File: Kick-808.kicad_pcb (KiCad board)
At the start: 2 copper layers, 19.3 x 106.5 mm, 70 parts, among them J3 Conn_02x05_Odd_Even, Q1 BC847, Q2 BC847, Q3 BC857, Q4 BC847, Q5 BC847, Q6 BC847, Q7 BC847, SW1 SW_Push_LED, U1 TL072, U2 TL072

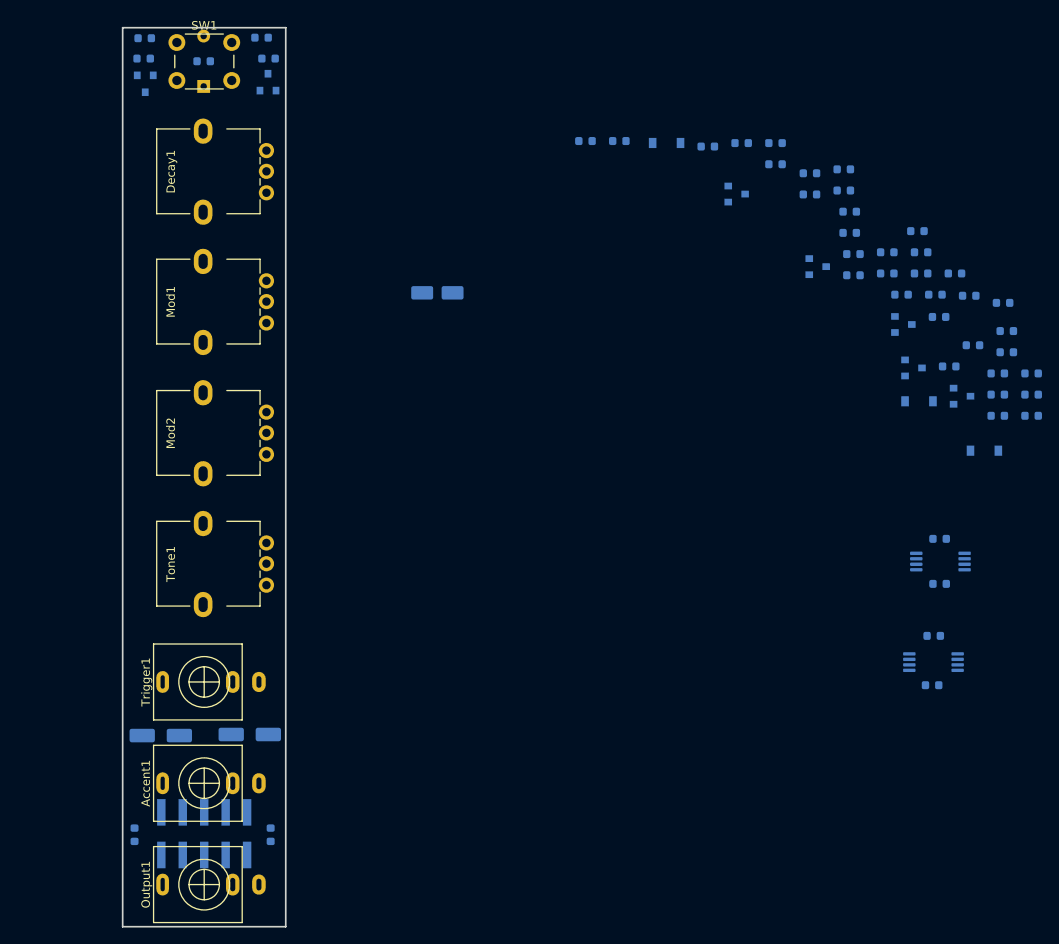
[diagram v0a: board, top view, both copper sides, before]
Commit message: Outline placement.
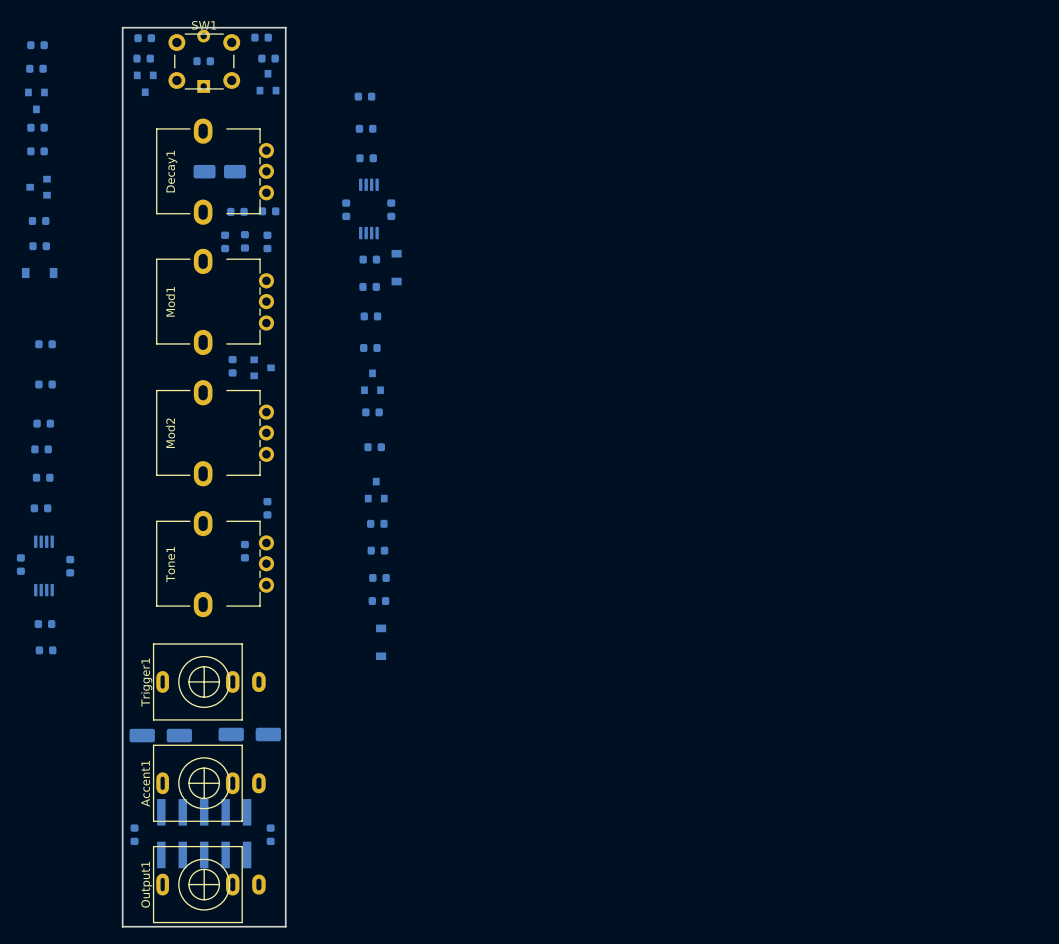
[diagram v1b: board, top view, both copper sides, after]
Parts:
- moved R15 119.8 mm to (107.4, 71.2), turned to 180 degrees
- moved R30 118.4 mm to (108.1, 119.0)
- moved R4 117.6 mm to (107.7, 98.3), turned to 180 degrees
- moved R11 116.5 mm to (107.7, 105.3)
- moved D2 113.9 mm to (107.5, 77.4)
- moved C2 111.0 mm to (107.3, 63.0), turned to 180 degrees
- moved R3 110.7 mm to (108.0, 95.2), turned to 180 degrees
- moved C14 108.9 mm to (105.3, 112.0), turned to 270 degrees
- moved R12 108.2 mm to (107.3, 60.2)
- moved U1 106.0 mm to (108.0, 112.1), turned to 270 degrees
- moved C11 105.5 mm to (108.3, 122.1), turned to 180 degrees
- moved C8 104.5 mm to (107.5, 74.2), turned to 180 degrees
- moved Q4 103.7 mm to (107.4, 67.2), turned to 180 degrees
- moved R8 103.1 mm to (107.1, 53.2), turned to 180 degrees
- moved C15 102.6 mm to (111.1, 112.1), turned to 270 degrees
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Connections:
- Accent1 pad S: GND -> (no net)
- C11 pad 2: GND -> (no net)
- C12 pad 2: GND -> (no net)
- C14 pad 1: GND -> (no net)
- C15 pad 2: GND -> (no net)
- C2 pad 2: GND -> (no net)
- C3 pad 2: GND -> (no net)
- C4 pad 1: GND -> (no net)
- C6 pad 1: GND -> (no net)
- C7 pad 2: GND -> (no net)
- D2 pad 1: GND -> (no net)
- D3 pad 2: GND -> (no net)
- J3 pad 3: GND -> (no net)
- J3 pad 4: GND -> (no net)
- J3 pad 5: GND -> (no net)
- J3 pad 6: GND -> (no net)
- J3 pad 7: GND -> (no net)
- J3 pad 8: GND -> (no net)
- Mod2 pad 2: GND -> (no net)
- Mod2 pad 3: GND -> (no net)
- Output1 pad S: GND -> (no net)
- Q1 pad 2: GND -> (no net)
- Q2 pad 2: GND -> (no net)
- Q4 pad 2: GND -> (no net)
- Q5 pad 2: GND -> (no net)
- Q7 pad 2: GND -> (no net)
- R10 pad 2: GND -> (no net)
- R17 pad 2: GND -> (no net)
- R2 pad 2: GND -> (no net)
- R27 pad 2: GND -> (no net)
- R5 pad 2: GND -> (no net)
- R6 pad 2: GND -> (no net)
- R8 pad 1: GND -> (no net)
- Trigger1 pad S: GND -> (no net)
